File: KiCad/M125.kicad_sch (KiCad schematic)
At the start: 9 parts, among them J1 Shelly, U1 ESP32-PICO-MINI-02

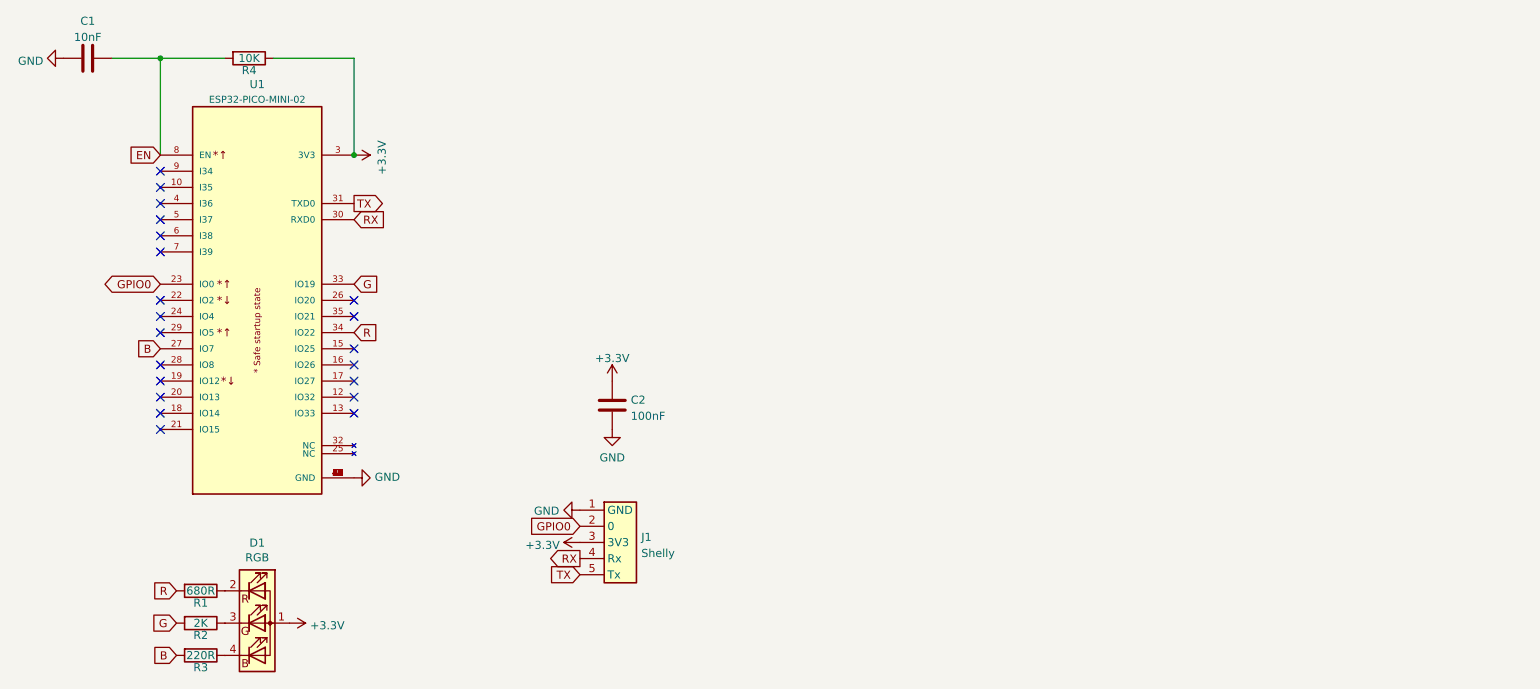
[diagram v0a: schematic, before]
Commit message: Tweak PCBs
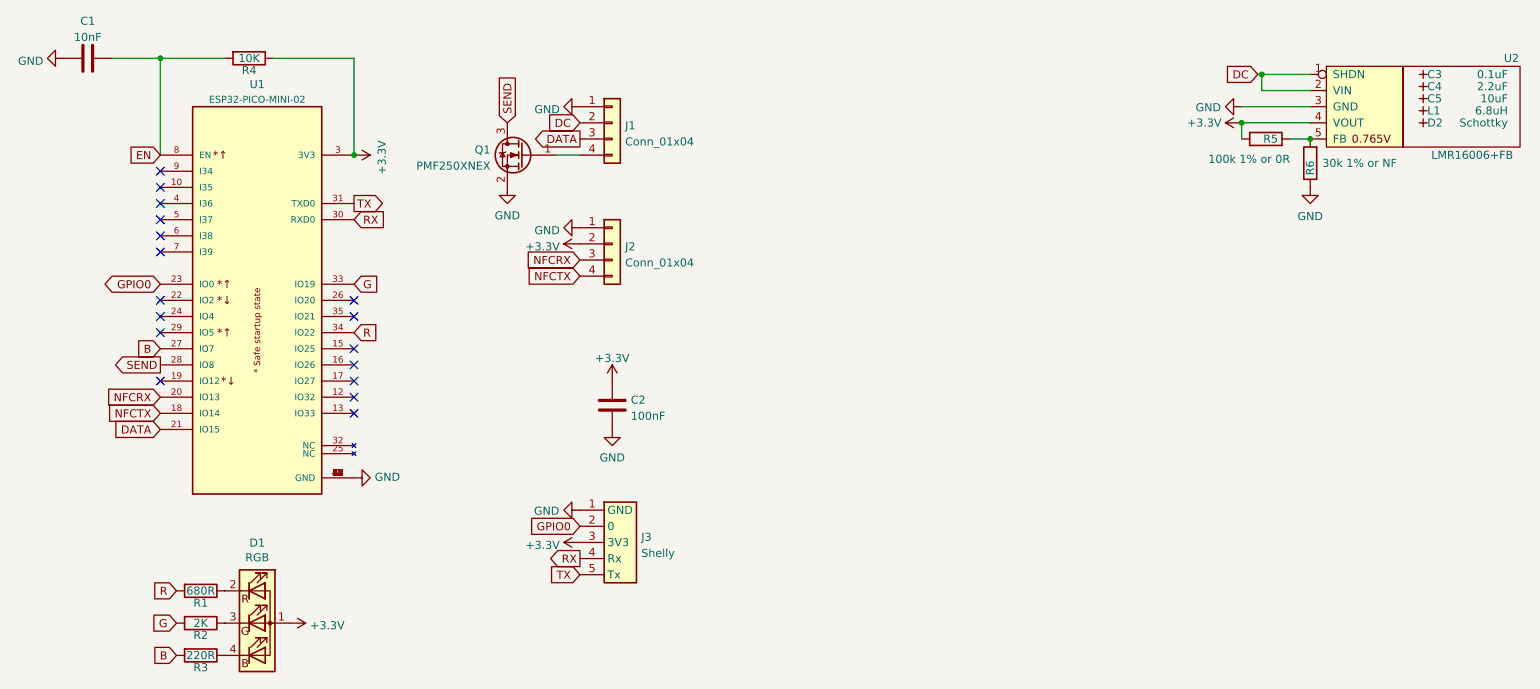
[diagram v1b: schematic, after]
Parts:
- added C3: 0.1uF, RevK:Hidden, symbol RevK:Hidden
- added C4: 2.2uF, RevK:Hidden, symbol RevK:Hidden
- added C5: 10uF, RevK:Hidden, symbol RevK:Hidden
- added D2: Schottky, RevK:Hidden, symbol RevK:Hidden
- added J1, J2: Conn_01x04, RevK:Molex_MiniSPOX_H4RA, symbol Connector_Generic:Conn_01x04
- added L1: 6.8uH, RevK:Hidden, symbol RevK:Hidden
- added Q1: PMF250XNEX, Package_TO_SOT_SMD:SOT-323_SC-70, symbol RevK:NX7002AK
- added R5: 100k 1% or 0R, RevK:R_0603, symbol Device:R
- added R6: 30k 1% or NF, RevK:R_0603, symbol Device:R
- added U2: LMR16006+FB, RevK:RegulatorBlockFB, symbol RevK:LMR16006+FB
- R4: footprint RevK:Pad_0603_Bridged -> RevK:R_0603
- renumbered J1 to J3
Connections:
- net +3V3: now also J2.2 (Pin_2), R5.1, U2.4 (VOUT)
- net GND: now also J1.1 (Pin_1), J2.1 (Pin_1), Q1.2 (S), R6.1, U2.3 (GND)
- net NFCTX: now reaches U1.18 (IO14)
- net NFCTX: now also J2.4 (Pin_4)
- net NFCRX: now reaches U1.20 (IO13)
- net NFCRX: now also J2.3 (Pin_3)
- net DATA: now reaches U1.21 (IO15)
- net DATA: now also J1.3 (Pin_3)
- net SEND: now reaches U1.28 (IO8)
- net SEND: now also Q1.3 (D)
- new net: J1.4 (Pin_4), Q1.1 (G)
- new net: R5.2, R6.2, U2.5 (FB)
- new net DC: J1.2 (Pin_2), U2.1 (SHDN), U2.2 (VIN)
- no-connect marks 21 -> 17
